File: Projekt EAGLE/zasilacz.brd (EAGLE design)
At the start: 152.4 x 121.6 mm, 91 parts, among them IC1 7805TV, IC3 7812TV, Q10 2N4126, Q11 2N4126, Q12 2N4126, Q13 2N4126, Q7 2N4126, Q9 2N4126, T1 2SC1815, U1 STM32L100C-DISCO, U2 IR2101, U3 IR2101, U4 IR2101, X1 22-23-2081, X2 22-23-2081

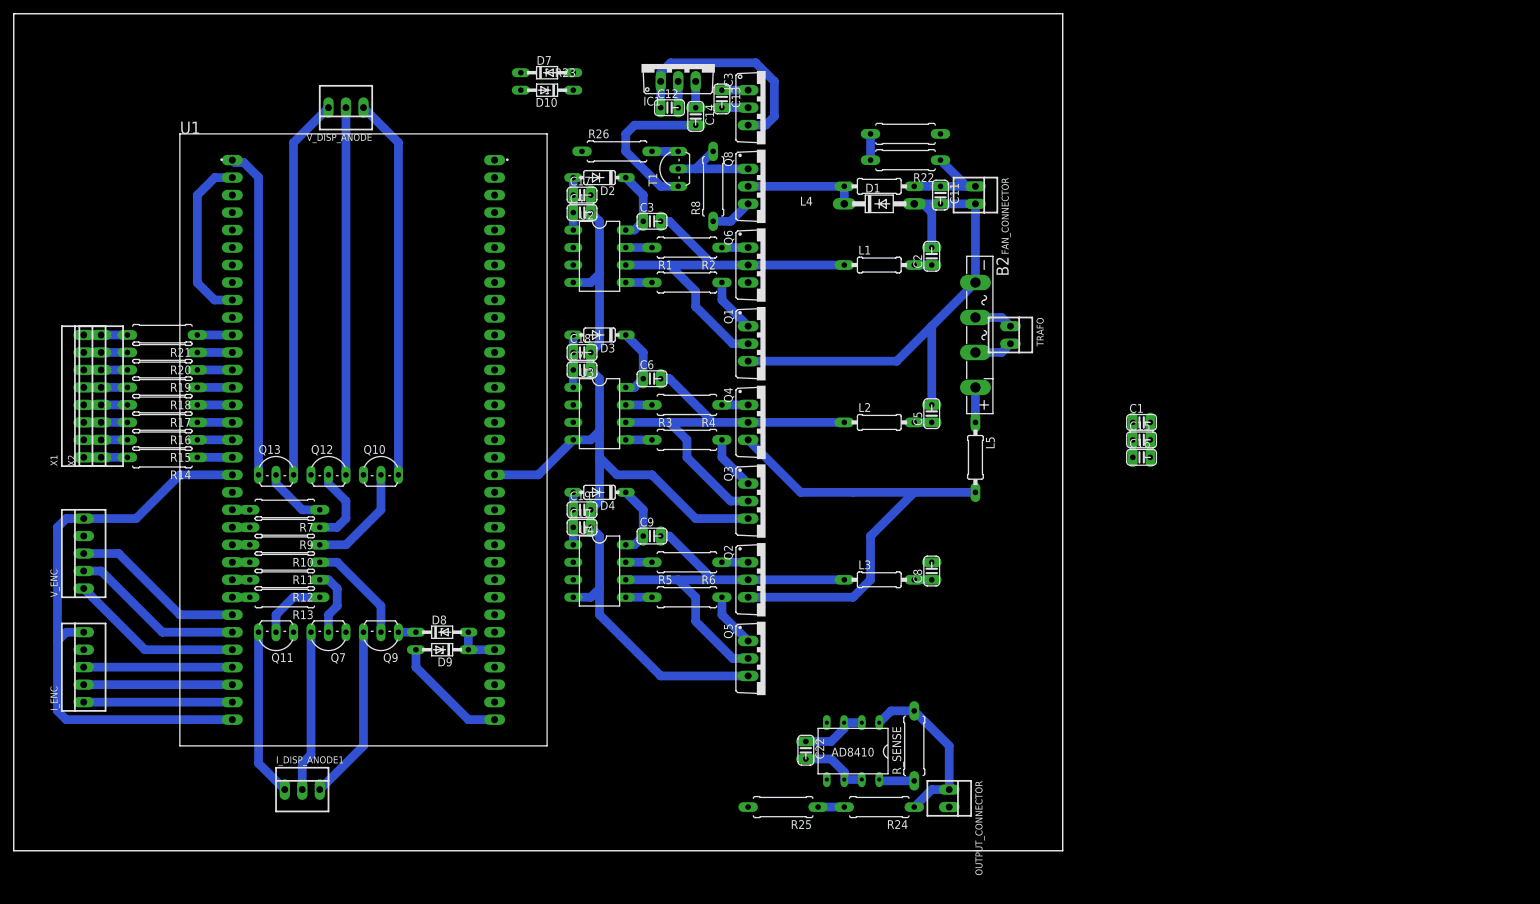
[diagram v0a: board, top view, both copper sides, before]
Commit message: Add files via upload
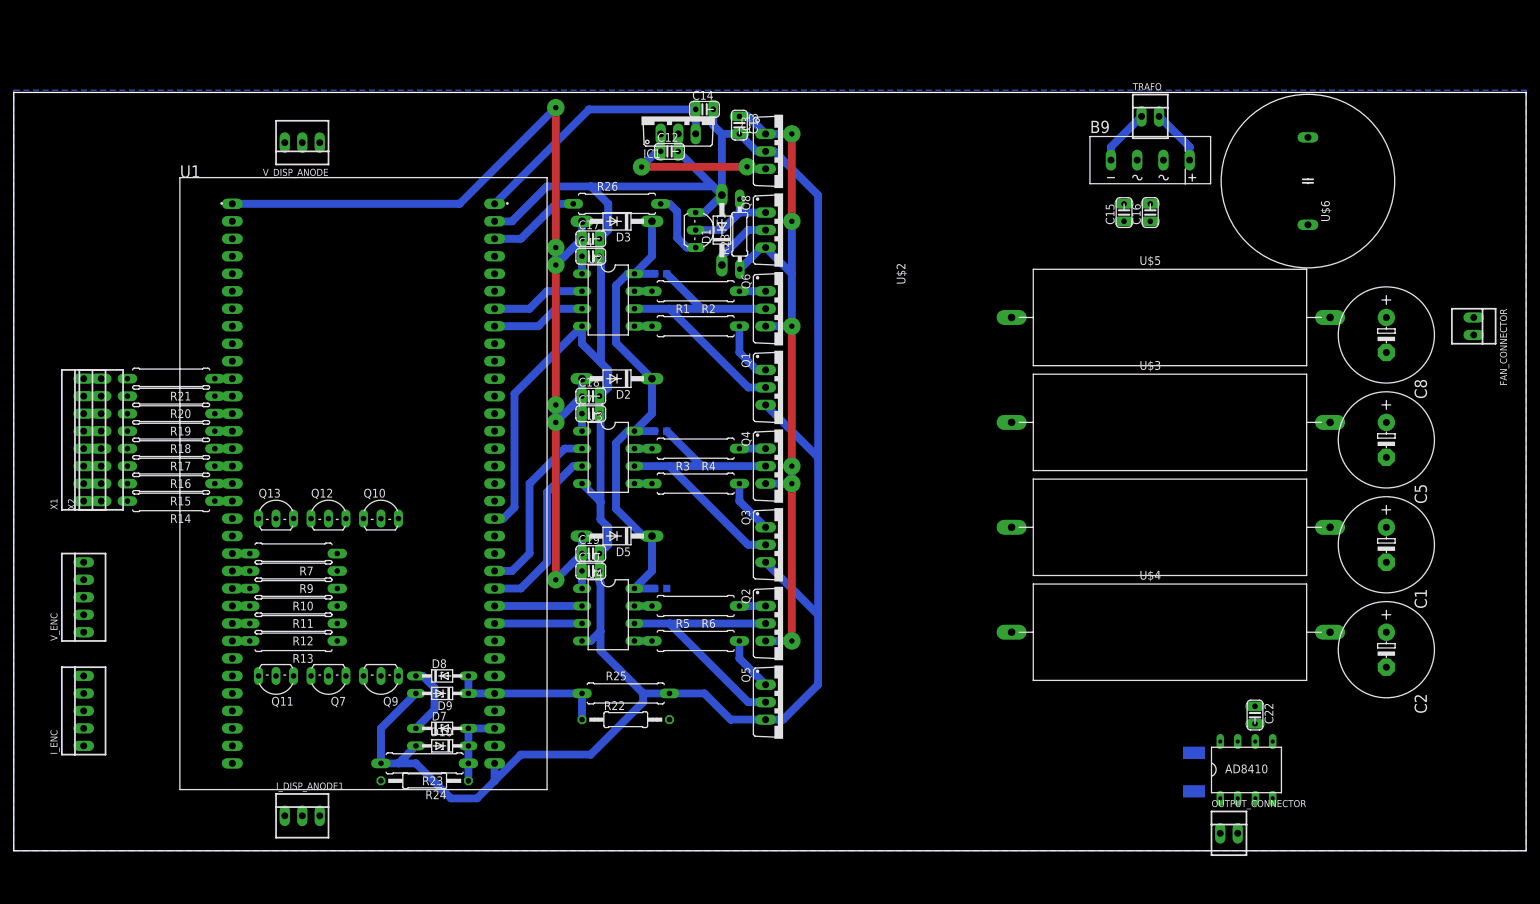
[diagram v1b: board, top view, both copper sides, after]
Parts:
- removed B2: (no value), rectifier:GBU4S
- removed C3, C6, C9: (no value), rcl:C025-024X044
- removed D4: (no value), diode:DO35-7
- removed L1, L2, L3, L4, L5: (no value), rcl:0207/10
- removed R8, R_SENSE: (no value), rcl:0309/10
- added B9: RECTIFIER-2KBP, rectifier:2KBP
- added C20, C21: (no value), rcl:C0603K
- added D5: SB120, diode:DO41-10
- added R27: (no value), rcl:R2512
- added R28: (no value), rcl:0207/10
- added U$2, U$3, U$4, U$5: 5256-RC5256-RC, rcl:INDAD4030W90L3300D1350B
- added U$6: C_MOJE_GRID12MM5, rcl:C025-030X050
- C1, C2, C5, C8: device rcl:C025-024X044 -> rcl:E5-13
- C11: device rcl:C025-024X044 -> rcl:C0603K
- D2, D3: value (none) -> SB120; device diode:DO35-7 -> diode:DO41-10
- R22, R24: device rcl:0309/10 -> rcl:0207/12
- moved R23 115.8 mm to (58.4, 12.7), turned to 180 degrees
- moved D10 96.5 mm to (62.2, 15.2)
- moved D7 96.5 mm to (62.2, 17.8)
- moved R22 90.9 mm to (88.9, 19.1), turned to 0 degrees
- moved C2 87.3 mm to (199.4, 29.2), turned to 270 degrees
- moved FAN_CONNECTOR 74.9 mm to (212.1, 76.2)
- moved C8 74.4 mm to (199.4, 74.9), turned to 270 degrees
- moved R24 66.1 mm to (59.7, 10.2)
- moved C5 66.1 mm to (199.4, 59.7), turned to 270 degrees
- moved C22 65.4 mm to (180.3, 19.7)
- moved U$1 47.9 mm to (174.0, 8.44), turned to 0 degrees
- moved C11 42.2 mm to (94.0, 83.8), flipped to the bottom, turned to 180 degrees
- moved OUTPUT_CONNECTOR 41.0 mm to (176.5, 2.54), turned to 0 degrees
- moved C1 39.8 mm to (199.4, 44.5), turned to 270 degrees
- moved TRAFO 37.7 mm to (165.1, 106.7), turned to 0 degrees
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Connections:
- removed net N$6: B2.+, L5.1
- net +R_SENSE: now also C1.+, C2.+, C5.+, R27.1, U$2.2, U$3.2, U$4.2; no longer C2.1, C5.1, C8.1, L1.2, L2.2, L3.2, R_SENSE.1
- net -R_SENSE: now also R22.2, R27.2; no longer R24.1, R_SENSE.2
- net 3V3: now also D5.A; no longer D4.A
- net FAN_PWM: now also U1.P2_3; no longer U1.P2_32
- net GND: now also B9.AC2, C1.-, C2.-, C5.-, C8.-, U$6.2; no longer B2.-, C1.1, C11.2, C2.2, C5.2, C8.2
- net N$1: now also R28.2; no longer R8.2
- net N$23: now also B9.+; no longer B2.AC1
- net N$27: now also B9.-; no longer B2.AC2
- net N$29: now also U$5.1; no longer L4.1
- net PH1VS: now also C11.2, U$3.1; no longer C3.2, L1.1
- net PH1_HIN: now also U1.P2_7; no longer U1.P2_20
- net PH1_LIN: now also U1.P2_8; no longer U1.P2_21
- net PH2VS: now also C20.2, U$2.1; no longer C6.2, L2.1
- net PH3VS: now also C21.2, U$4.1; no longer C9.2, L3.1
- net UWY: now also C8.+, R24.2, U$5.2; no longer C11.1, L4.2, R22.1
- net VB: now also C11.1, C20.1, C21.1, D5.C; no longer C3.1, C6.1, C9.1, D4.C
- net VCC: now also B9.AC1, R28.1, U$6.1; no longer C1.2, L5.2, R8.1
- net V_MEASURE_FAN: now also R24.1; no longer R22.2
- net V_MEASURE_OUT: now also R22.1; no longer R24.2
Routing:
- net 3V3: track 73.5 -> 170.8 mm, vias 0 -> 6
- net N$37: track 55.4 -> 0.00 mm
- net N$21: track 55.4 -> 0.00 mm
- net N$32: track 53.3 -> 0.00 mm
- net VB: track 31.4 -> 73.7 mm
- net 5V: track 3.81 -> 38.5 mm
- net PH2_LIN: track 0.00 -> 26.0 mm
- net PH2_HIN: track 0.00 -> 26.0 mm
- net N$42: track 25.5 -> 0.00 mm
- net -R_SENSE: track 25.5 -> 0.00 mm
- net N$59: track 25.3 -> 0.00 mm
- net N$58: track 25.3 -> 0.00 mm
- net N$57: track 25.3 -> 0.00 mm
- net N$44: track 24.4 -> 0.00 mm
- net N$43: track 23.4 -> 0.00 mm
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- added copper zone on layer 16, net GND
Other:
- board size 152.4 x 121.6 mm -> 219.7 x 110.2 mm
